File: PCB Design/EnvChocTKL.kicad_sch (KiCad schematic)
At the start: 192 parts, among them J1 Type-c-31-m-14, SW101 EVQPU, SW102 EVQPU

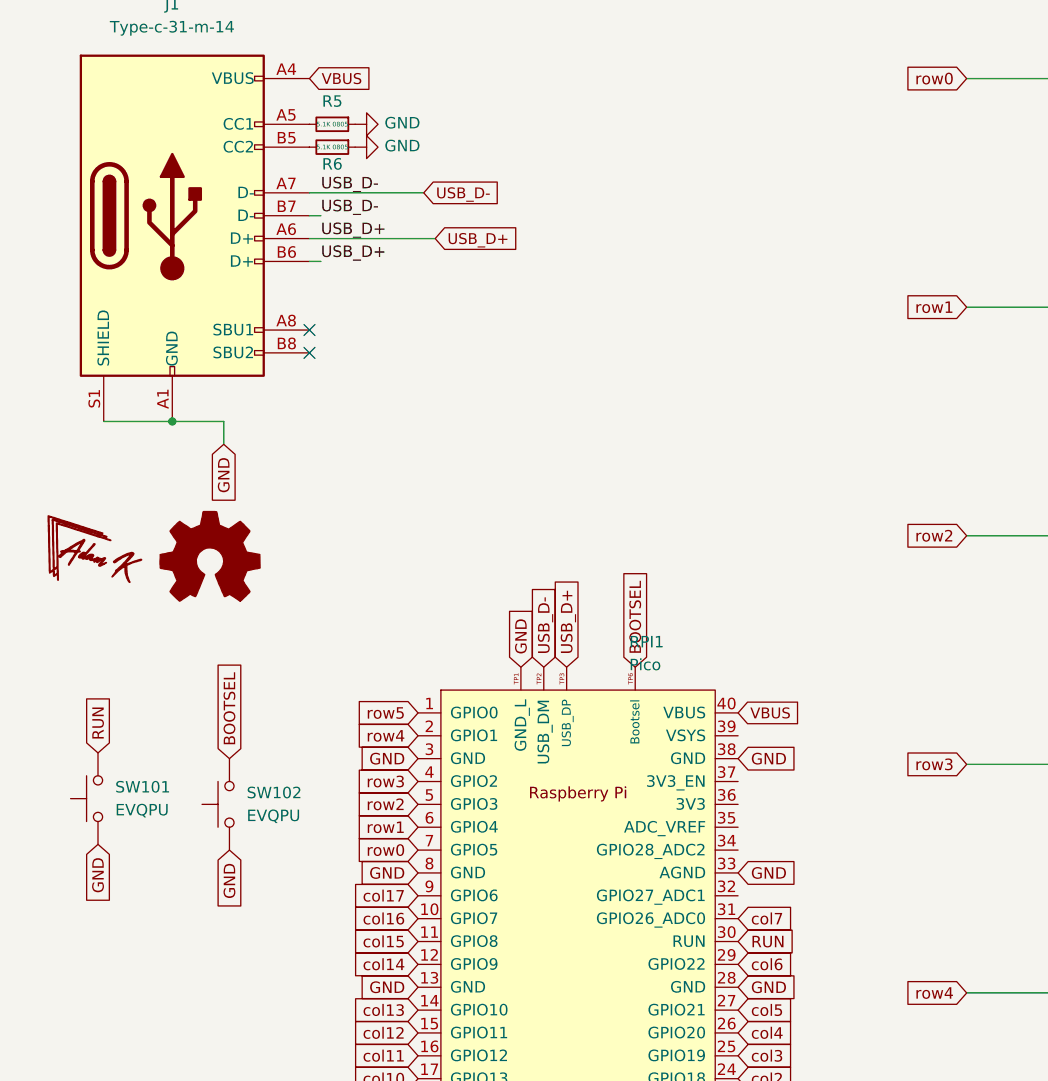
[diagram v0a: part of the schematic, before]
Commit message: checks and preparation to order
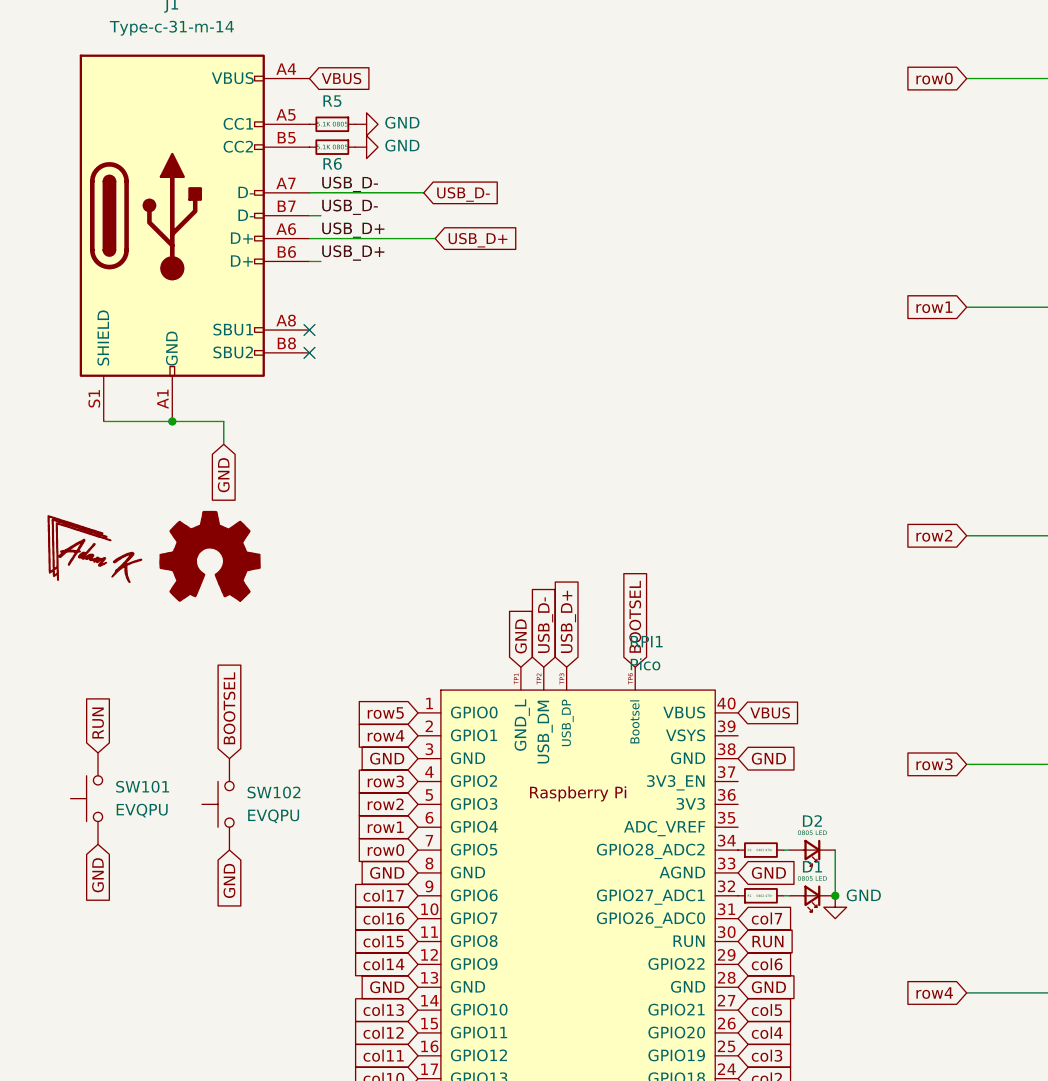
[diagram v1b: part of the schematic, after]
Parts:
- added D1, D2: 0805 LED, LED_SMD:LED_0805_2012Metric, symbol Device:LED_Small
- added R1, R2: 0402 470r, Resistor_SMD:R_0402_1005Metric, symbol Device:R_Small
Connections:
- net GND: now also D1.1 (K), D2.1 (K)
- net at RPI1.32 (GPIO27_ADC1): now also R1.1
- net at RPI1.34 (GPIO28_ADC2): now also R2.1
- new net: D1.2 (A), R1.2
- new net: D2.2 (A), R2.2
